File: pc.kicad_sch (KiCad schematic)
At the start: 6 parts

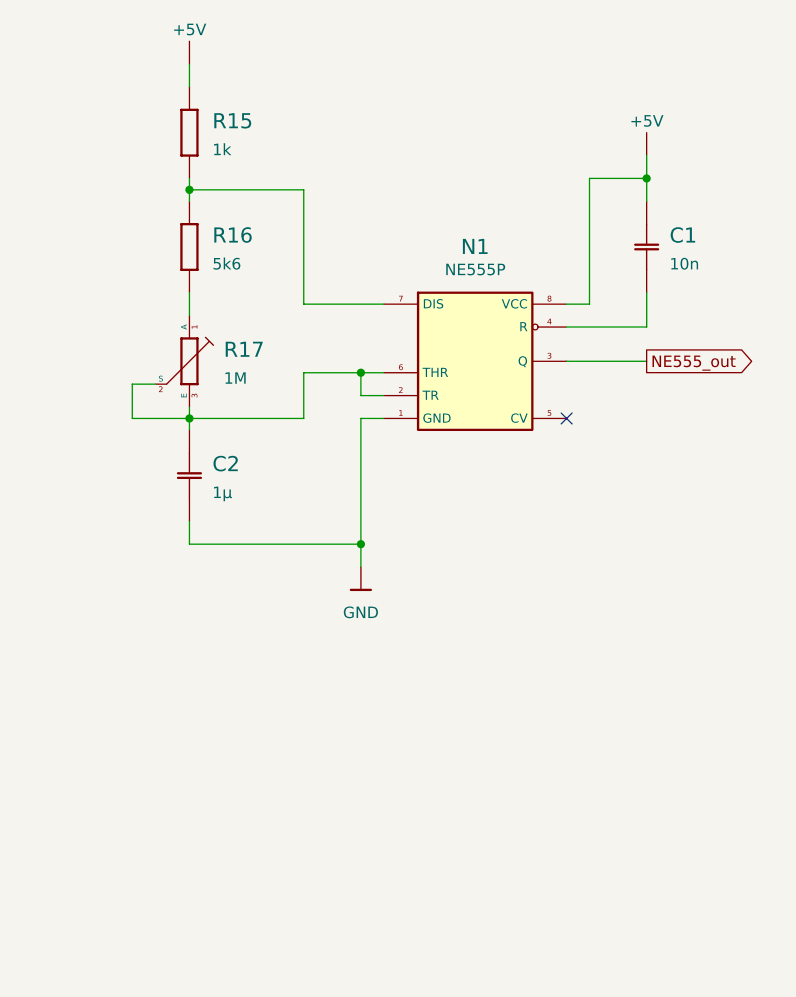
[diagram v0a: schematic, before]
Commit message: addes pc sim + kicad fix
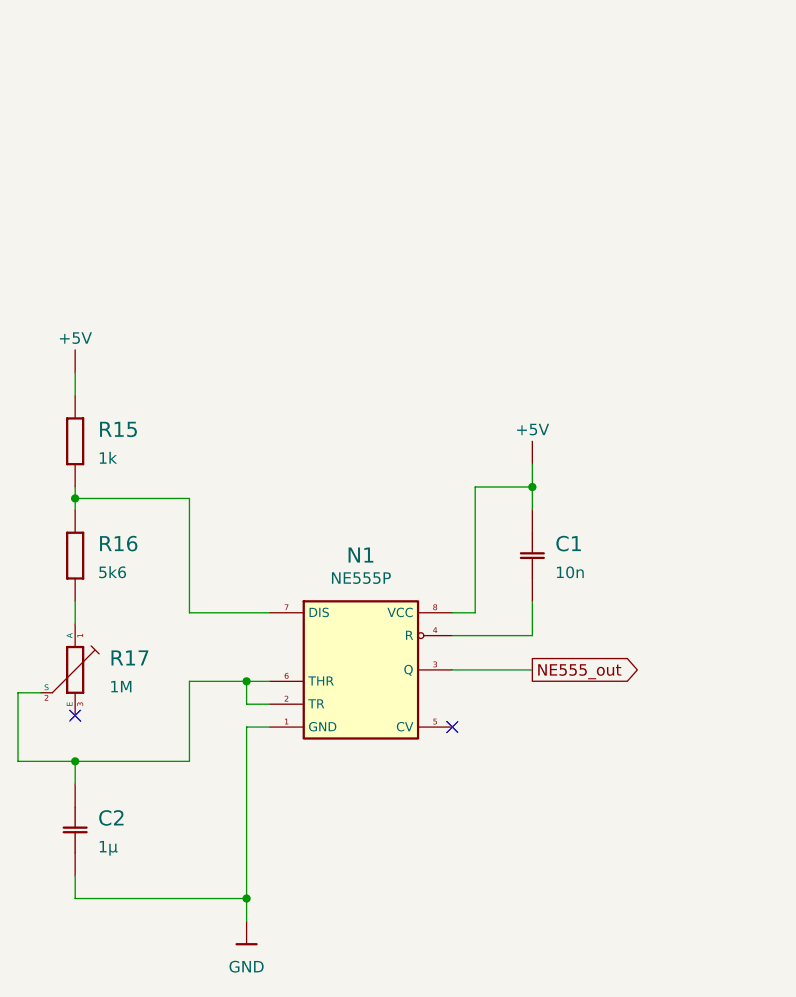
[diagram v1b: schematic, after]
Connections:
- net at C2.2, N1.2 (TR), N1.6 (THR)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: no longer R17.3 (E)
- no-connect marks 1 -> 2
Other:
- moved on the sheet: C1, C2, N1, R15, R16, R17
